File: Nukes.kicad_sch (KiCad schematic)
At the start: 25 parts, among them J6 Screw_Terminal_01x08, J7 Conn_01x05_Male, Q2 NCV8415STT1G, Q3 NCV8415STT1G, Q4 NCV8415STT1G, Q5 NCV8415STT1G, U3 LTV-247, U4 PCA9534RGVR, U5 PCA9685BS

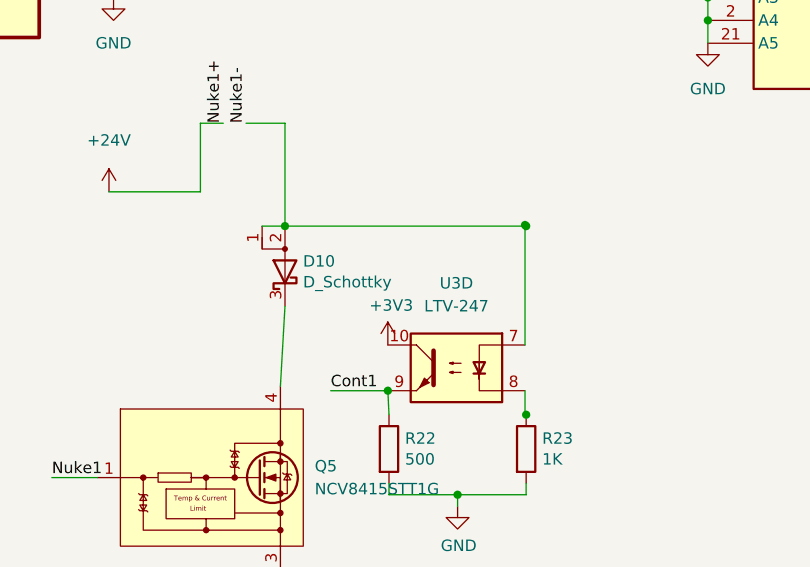
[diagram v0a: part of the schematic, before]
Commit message: made more progress
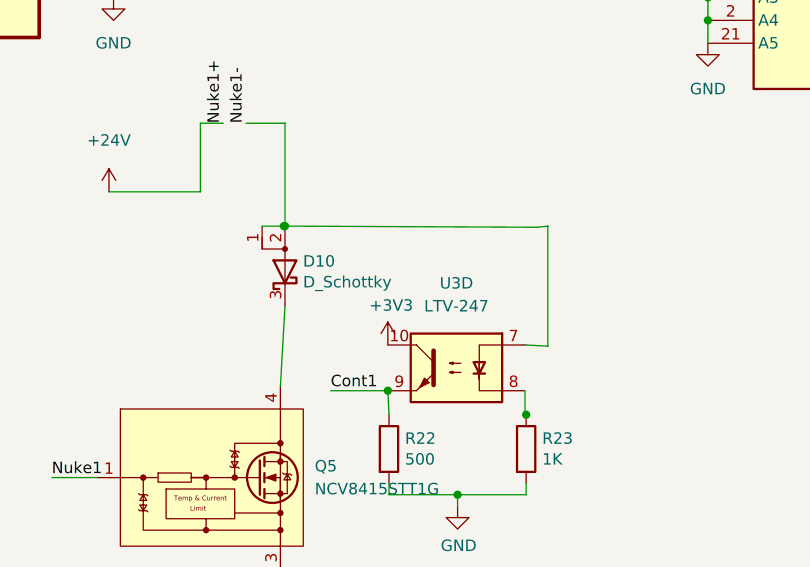
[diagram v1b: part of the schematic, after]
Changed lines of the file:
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@@
   (junction (at 60.96 113.03) (diameter 0) (color 0 0 0 0)
   )
+  (junction (at 119.253 92.71) (diameter 0) (color 0 0 0 0)
+  )
   (junction (at 67.056 150.495) (diameter 0) (color 0 0 0 0)
   )
   (junction (at 184.15 20.32) (diameter 0) (color 0 0 0 0)
   )
-  (junction (at 146.177 92.71) (diameter 0) (color 0 0 0 0)
-  )
   (junction (at 39.37 149.86) (diameter 0) (color 0 0 0 0)
   )
@@
   )
   (junction (at 166.37 64.77) (diameter 0) (color 0 0 0 0)
-  )
-  (junction (at 146.05 92.583) (diameter 0) (color 0 0 0 0)
   )
   (junction (at 146.177 113.665) (diameter 0) (color 0 0 0 0)
@@
     (stroke (width 0) (type default) (color 0 0 0 0))
   )
+  (wire (pts (xy 119.38 92.71) (xy 147.447 92.837))
+    (stroke (width 0) (type default) (color 0 0 0 0))
+  )
   (wire (pts (xy 39.37 161.29) (xy 39.37 167.64))
     (stroke (width 0) (type default) (color 0 0 0 0))
@@
     (stroke (width 0) (type default) (color 0 0 0 0))
   )
-  (wire (pts (xy 116.84 92.71) (xy 119.38 92.71))
+  (wire (pts (xy 116.84 92.71) (xy 119.253 92.71))
     (stroke (width 0) (type default) (color 0 0 0 0))
   )
@@
     (stroke (width 0) (type default) (color 0 0 0 0))
   )
+  (wire (pts (xy 119.253 92.71) (xy 119.38 92.71))
+    (stroke (width 0) (type default) (color 0 0 0 0))
+  )
   (wire (pts (xy 50.8 48.895) (xy 61.595 48.895))
     (stroke (width 0) (type default) (color 0 0 0 0))
@@
     (stroke (width 0) (type default) (color 0 0 0 0))
   )
+  (wire (pts (xy 148.59 106.045) (xy 146.05 105.918))
+    (stroke (width 0) (type default) (color 0 0 0 0))
+  )
   (wire (pts (xy 119.38 81.28) (xy 119.38 92.71))
     (stroke (width 0) (type default) (color 0 0 0 0))
@@
     (stroke (width 0) (type default) (color 0 0 0 0))
   )
-  (wire (pts (xy 146.05 92.583) (xy 146.177 92.71))
+  (wire (pts (xy 148.59 92.71) (xy 147.447 92.837))
     (stroke (width 0) (type default) (color 0 0 0 0))
   )
@@
     (stroke (width 0) (type default) (color 0 0 0 0))
   )
-  (wire (pts (xy 119.38 92.71) (xy 146.177 92.71))
-    (stroke (width 0) (type default) (color 0 0 0 0))
-  )
   (wire (pts (xy 98.552 120.65) (xy 93.472 120.65))
     (stroke (width 0) (type default) (color 0 0 0 0))
@@
     (stroke (width 0) (type default) (color 0 0 0 0))
   )
-  (wire (pts (xy 146.05 92.583) (xy 146.05 105.918))
-    (stroke (width 0) (type default) (color 0 0 0 0))
-  )
+  (wire (pts (xy 148.59 92.71) (xy 148.59 106.045))
+    (stroke (width 0) (type default) (color 0 0 0 0))
+  )
